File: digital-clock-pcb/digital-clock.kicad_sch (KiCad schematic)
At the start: 31 parts, among them J1 USB_OTG, J2 Conn_02x03_Odd_Even, J3 Conn_01x04, J4 Conn_01x04, U1 ATmega328P-M, U2 PCF8523T, Y1 ABS2532768KHZ6T

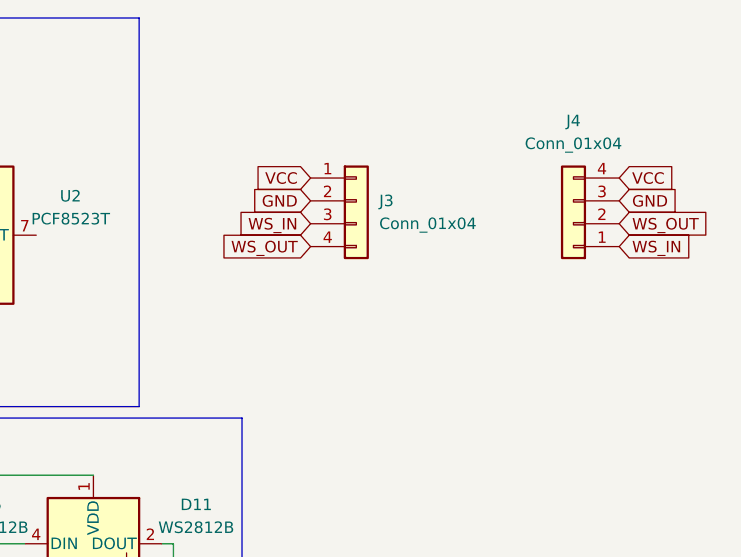
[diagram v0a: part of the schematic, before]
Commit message: wiring connector
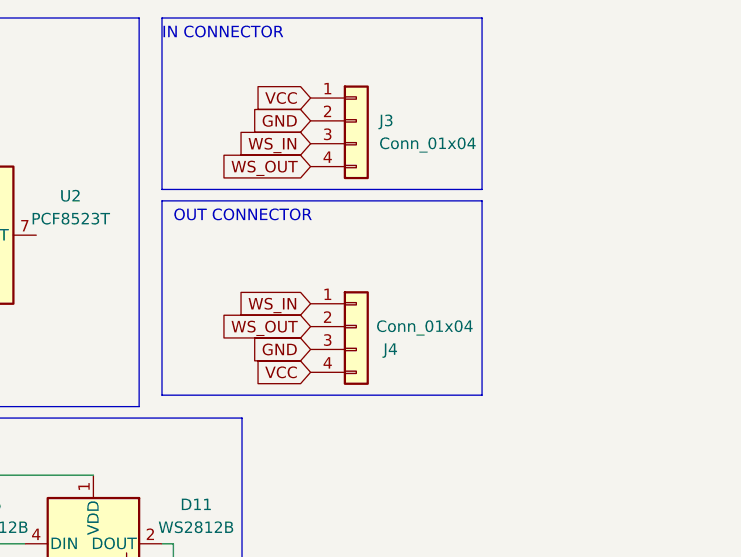
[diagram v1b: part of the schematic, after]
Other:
- note added: "IN CONNECTOR"
- note added: "OUT CONNECTOR"
- moved on the sheet: J3, J4
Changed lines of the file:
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@@
+    (stroke (width 0) (type default) (color 0 0 0 0))
+  )
+  (polyline (pts (xy 144.78 34.29) (xy 144.78 55.88))
     (stroke (width 0) (type default) (color 0 0 0 0))
   )
@@
     (stroke (width 0) (type default) (color 0 0 0 0))
   )
+  (polyline (pts (xy 144.78 34.29) (xy 180.34 34.29))
+    (stroke (width 0) (type default) (color 0 0 0 0))
+  )
   (wire (pts (xy 78.74 115.57) (xy 78.74 133.35))
     (stroke (width 0) (type default) (color 0 0 0 0))
   )
+  (polyline (pts (xy 180.34 33.02) (xy 144.78 33.02))
+    (stroke (width 0) (type default) (color 0 0 0 0))
+  )
   (wire (pts (xy 144.78 72.39) (xy 146.05 72.39))
     (stroke (width 0) (type default) (color 0 0 0 0))
@@
     (stroke (width 0) (type default) (color 0 0 0 0))
   )
+  (polyline (pts (xy 144.78 13.97) (xy 144.78 33.02))
+    (stroke (width 0) (type default) (color 0 0 0 0))
+  )
   (wire (pts (xy 93.98 33.02) (xy 99.06 33.02))
     (stroke (width 0) (type default) (color 0 0 0 0))
@@
     (stroke (width 0) (type default) (color 0 0 0 0))
   )
+  (polyline (pts (xy 144.78 13.97) (xy 180.34 13.97))
+    (stroke (width 0) (type default) (color 0 0 0 0))
+  )
   (wire (pts (xy 147.32 170.18) (xy 81.28 170.18))
     (stroke (width 0) (type default) (color 0 0 0 0))
@@
     (stroke (width 0) (type default) (color 0 0 0 0))
   )
+  (polyline (pts (xy 180.34 13.97) (xy 180.34 33.02))
+    (stroke (width 0) (type default) (color 0 0 0 0))
+  )
   (polyline (pts (xy 142.24 13.97) (xy 81.28 13.97))
     (stroke (width 0) (type default) (color 0 0 0 0))
@@
     (stroke (width 0) (type default) (color 0 0 0 0))
   )
+  (polyline (pts (xy 180.34 34.29) (xy 180.34 55.88))
+    (stroke (width 0) (type default) (color 0 0 0 0))
+  )
   (wire (pts (xy 91.44 135.89) (xy 73.66 135.89))
     (stroke (width 0) (type default) (color 0 0 0 0))
@@
     (stroke (width 0) (type default) (color 0 0 0 0))
   )
+  (polyline (pts (xy 180.34 55.88) (xy 144.78 55.88))
+    (stroke (width 0) (type default) (color 0 0 0 0))
+  )
   (wire (pts (xy 78.74 133.35) (xy 78.74 151.13))
     (stroke (width 0) (type default) (color 0 0 0 0))
@@
   (wire (pts (xy 83.82 46.99) (xy 83.82 40.64))
     (stroke (width 0) (type default) (color 0 0 0 0))
+  )
+  (text "IN CONNECTOR" (at 144.78 16.51 0)
+    (effects (font (size 1.27 1.27)) (justify left bottom))
+  )
+  (text "OUT CONNECTOR" (at 146.05 36.83 0)
+    (effects (font (size 1.27 1.27)) (justify left bottom))
   )
   (text "RTC PCF8523" (at 81.28 16.51 0)
@@
     )
   )
-  (global_label "VCC" (shape input) (at 195.58 31.75 0) (fields_autoplaced)
-    (effects (font (size 1.27 1.27)) (justify left))
-    (property "Intersheet References" "${INTERSHEET_REFS}" (id 0) (at 201.6217 31.6706 0)
-      (effects (font (size 1.27 1.27)) (justify left) hide)
+  (global_label "VCC" (shape input) (at 161.29 53.34 180) (fields_autoplaced)
+    (effects (font (size 1.27 1.27)) (justify right))
+    (property "Intersheet References" "${INTERSHEET_REFS}" (id 0) (at 155.2483 53.4194 0)
+      (effects (font (size 1.27 1.27)) (justify right) hide)
     )
   )
@@
     )
   )
-  (global_label "VCC" (shape input) (at 161.29 31.75 180) (fields_autoplaced)
-    (effects (font (size 1.27 1.27)) (justify right))
-    (property "Intersheet References" "${INTERSHEET_REFS}" (id 0) (at 155.2483 31.6706 0)
+  (global_label "VCC" (shape input) (at 161.29 22.86 180) (fields_autoplaced)
+    (effects (font (size 1.27 1.27)) (justify right))
+    (property "Intersheet References" "${INTERSHEET_REFS}" (id 0) (at 155.2483 22.7806 0)
       (effects (font (size 1.27 1.27)) (justify right) hide)
     )
@@
     )
   )
-  (global_label "WS_IN" (shape input) (at 195.58 39.37 0) (fields_autoplaced)
-    (effects (font (size 1.27 1.27)) (justify left))
-    (property "Intersheet References" "${INTERSHEET_REFS}" (id 0) (at 203.5569 39.2906 0)
-      (effects (font (size 1.27 1.27)) (justify left) hide)
+  (global_label "WS_IN" (shape input) (at 161.29 45.72 180) (fields_autoplaced)
+    (effects (font (size 1.27 1.27)) (justify right))
+    (property "Intersheet References" "${INTERSHEET_REFS}" (id 0) (at 153.3131 45.7994 0)
+      (effects (font (size 1.27 1.27)) (justify right) hide)
     )
   )
@@
     )
   )
-  (global_label "WS_IN" (shape input) (at 161.29 36.83 180) (fields_autoplaced)
-    (effects (font (size 1.27 1.27)) (justify right))
-    (property "Intersheet References" "${INTERSHEET_REFS}" (id 0) (at 153.3131 36.7506 0)
+  (global_label "WS_IN" (shape input) (at 161.29 27.94 180) (fields_autoplaced)
+    (effects (font (size 1.27 1.27)) (justify right))
+    (property "Intersheet References" "${INTERSHEET_REFS}" (id 0) (at 153.3131 27.8606 0)
       (effects (font (size 1.27 1.27)) (justify right) hide)
     )
@@
     )
   )
-  (global_label "WS_OUT" (shape input) (at 195.58 36.83 0) (fields_autoplaced)
-    (effects (font (size 1.27 1.27)) (justify left))
-    (property "Intersheet References" "${INTERSHEET_REFS}" (id 0) (at 205.2502 36.7506 0)
-      (effects (font (size 1.27 1.27)) (justify left) hide)
-    )
-  )
-  (global_label "GND" (shape input) (at 161.29 34.29 180) (fields_autoplaced)
-    (effects (font (size 1.27 1.27)) (justify right))
-    (property "Intersheet References" "${INTERSHEET_REFS}" (id 0) (at 155.0064 34.2106 0)
+  (global_label "WS_OUT" (shape input) (at 161.29 48.26 180) (fields_autoplaced)
+    (effects (font (size 1.27 1.27)) (justify right))
+    (property "Intersheet References" "${INTERSHEET_REFS}" (id 0) (at 151.6198 48.3394 0)
+      (effects (font (size 1.27 1.27)) (justify right) hide)
+    )
+  )
+  (global_label "GND" (shape input) (at 161.29 25.4 180) (fields_autoplaced)
+    (effects (font (size 1.27 1.27)) (justify right))
+    (property "Intersheet References" "${INTERSHEET_REFS}" (id 0) (at 155.0064 25.3206 0)
       (effects (font (size 1.27 1.27)) (justify right) hide)
     )
@@
     )
   )
-  (global_label "WS_OUT" (shape input) (at 161.29 39.37 180) (fields_autoplaced)
-    (effects (font (size 1.27 1.27)) (justify right))
-    (property "Intersheet References" "${INTERSHEET_REFS}" (id 0) (at 151.6198 39.2906 0)
+  (global_label "WS_OUT" (shape input) (at 161.29 30.48 180) (fields_autoplaced)
+    (effects (font (size 1.27 1.27)) (justify right))
+    (property "Intersheet References" "${INTERSHEET_REFS}" (id 0) (at 151.6198 30.4006 0)
       (effects (font (size 1.27 1.27)) (justify right) hide)
     )
@@
     )
   )
-  (global_label "GND" (shape input) (at 195.58 34.29 0) (fields_autoplaced)
-    (effects (font (size 1.27 1.27)) (justify left))
-    (property "Intersheet References" "${INTERSHEET_REFS}" (id 0) (at 201.8636 34.2106 0)
-      (effects (font (size 1.27 1.27)) (justify left) hide)
+  (global_label "GND" (shape input) (at 161.29 50.8 180) (fields_autoplaced)
+    (effects (font (size 1.27 1.27)) (justify right))
+    (property "Intersheet References" "${INTERSHEET_REFS}" (id 0) (at 155.0064 50.8794 0)
+      (effects (font (size 1.27 1.27)) (justify right) hide)
     )
   )
@@
     (pin "4")
   )
-  (symbol (lib_id "Connector_Generic:Conn_01x04") (at 166.37 34.29 0) (unit 1)
-    (in_bom yes) (on_board yes) (fields_autoplaced)
-    (property "Reference" "J3" (id 0) (at 168.91 34.2899 0)
+  (symbol (lib_id "Connector_Generic:Conn_01x04") (at 166.37 25.4 0) (unit 1)
+    (in_bom yes) (on_board yes) (fields_autoplaced)
+    (property "Reference" "J3" (id 0) (at 168.91 25.3999 0)
       (effects (font (size 1.27 1.27)) (justify left))
     )
-    (property "Value" "Conn_01x04" (id 1) (at 168.91 36.8299 0)
+    (property "Value" "Conn_01x04" (id 1) (at 168.91 27.9399 0)
       (effects (font (size 1.27 1.27)) (justify left))
     )
-    (property "Footprint" "Connector_JST:JST_SH_SM04B-SRSS-TB_1x04-1MP_P1.00mm_Horizontal" (id 2) (at 166.37 34.29 0)
+    (property "Footprint" "Connector_JST:JST_SH_SM04B-SRSS-TB_1x04-1MP_P1.00mm_Horizontal" (id 2) (at 166.37 25.4 0)
       (effects (font (size 1.27 1.27)) hide)
     )
-    (property "Datasheet" "~" (id 3) (at 166.37 34.29 0)
+    (property "Datasheet" "~" (id 3) (at 166.37 25.4 0)
       (effects (font (size 1.27 1.27)) hide)
     )
@@
     (pin "4")
   )
-  (symbol (lib_id "Connector_Generic:Conn_01x04") (at 190.5 36.83 180) (unit 1)
-    (in_bom yes) (on_board yes) (fields_autoplaced)
-    (property "Reference" "J4" (id 0) (at 190.5 25.4 0))
-    (property "Value" "Conn_01x04" (id 1) (at 190.5 27.94 0))
-    (property "Footprint" "Connector_JST:JST_SH_SM04B-SRSS-TB_1x04-1MP_P1.00mm_Horizontal" (id 2) (at 190.5 36.83 0)
+  (symbol (lib_id "Connector_Generic:Conn_01x04") (at 166.37 48.26 0) (unit 1)
+    (in_bom yes) (on_board yes)
+    (property "Reference" "J4" (id 0) (at 170.18 50.8 0))
+    (property "Value" "Conn_01x04" (id 1) (at 173.99 48.26 0))
+    (property "Footprint" "Connector_JST:JST_SH_SM04B-SRSS-TB_1x04-1MP_P1.00mm_Horizontal" (id 2) (at 166.37 48.26 0)
       (effects (font (size 1.27 1.27)) hide)
     )
-    (property "Datasheet" "~" (id 3) (at 190.5 36.83 0)
+    (property "Datasheet" "~" (id 3) (at 166.37 48.26 0)
       (effects (font (size 1.27 1.27)) hide)
     )

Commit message: change m328 package
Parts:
- U1: footprint Package_DFN_QFN:QFN-32-1EP_5x5mm_P0.5mm_EP3.1x3.1mm -> Package_QFP:TQFP-32_7x7mm_P0.8mm
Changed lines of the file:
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@@
       (effects (font (size 1.27 1.27)) (justify left))
     )
-    (property "Footprint" "Package_DFN_QFN:QFN-32-1EP_5x5mm_P0.5mm_EP3.1x3.1mm" (id 2) (at 35.56 99.06 0)
+    (property "Footprint" "Package_QFP:TQFP-32_7x7mm_P0.8mm" (id 2) (at 35.56 99.06 0)
       (effects (font (size 1.27 1.27) italic) hide)
     )
@@
     )
     (path "/ebd1509e-daba-42cf-8f1c-294b259f2169"
-      (reference "U1") (unit 1) (value "ATmega328P-M") (footprint "Package_DFN_QFN:QFN-32-1EP_5x5mm_P0.5mm_EP3.1x3.1mm")
+      (reference "U1") (unit 1) (value "ATmega328P-M") (footprint "Package_QFP:TQFP-32_7x7mm_P0.8mm")
     )
     (path "/d7af507e-f887-4995-925b-7c5f77d83df7"
